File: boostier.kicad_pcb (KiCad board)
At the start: 2 copper layers, 7 parts, among them U1 TLV61070ADBV, U2 SN74LV1T126DBVR

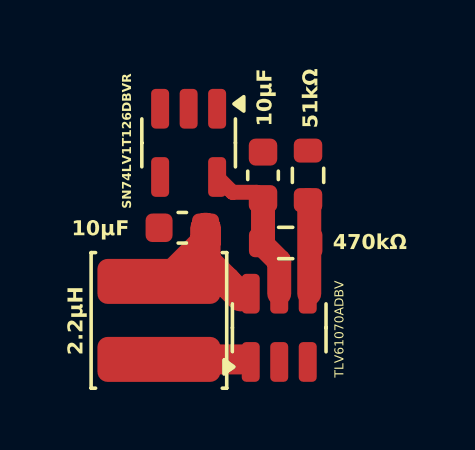
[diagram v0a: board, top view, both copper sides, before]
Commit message: Cleanup.
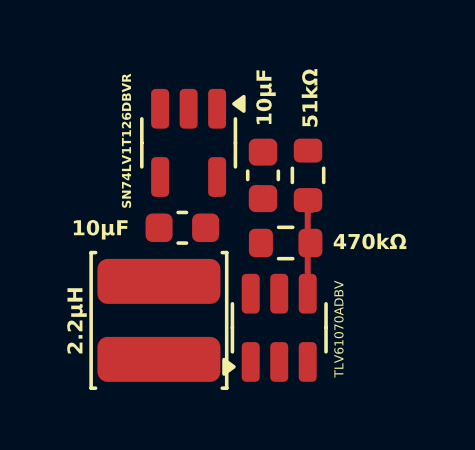
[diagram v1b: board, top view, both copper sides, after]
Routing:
- net RAW: track 7.58 -> 0.24 mm
- net 5V: track 5.28 -> 0.30 mm
- net BOOST_SW: track 2.75 -> 0.00 mm
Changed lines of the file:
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@@
-	)
-	(segment
-		(start 159.1025 98.97)
-		(end 160.415 97.6575)
-		(width 1)
-		(layer "F.Cu")
-		(net 1)
-	)
-	(segment
-		(start 158.86 98.97)
-		(end 161.09 98.97)
-		(width 1)
-		(layer "F.Cu")
-		(net 1)
-	)
-	(segment
-		(start 160.415 98.295)
-		(end 161.09 98.97)
-		(width 1)
-		(layer "F.Cu")
-		(net 1)
 	)
 	(segment
@@
 	)
 	(segment
-		(start 161.09 98.97)
-		(end 161.59 99.47)
-		(width 1)
-		(layer "F.Cu")
-		(net 1)
-	)
-	(segment
-		(start 160.415 97.6575)
-		(end 160.415 97.1825)
-		(width 1)
-		(layer "F.Cu")
-		(net 1)
-	)
-	(segment
-		(start 160.415 97.1825)
-		(end 160.415 98.295)
-		(width 1)
-		(layer "F.Cu")
-		(net 1)
-	)
-	(segment
-		(start 160.8 95.49)
-		(end 161.31 96)
-		(width 0.5)
-		(layer "F.Cu")
-		(net 3)
-	)
-	(segment
-		(start 162.33 97.62)
-		(end 162.26 97.69)
-		(width 0.8)
-		(layer "F.Cu")
-		(net 3)
-	)
-	(segment
-		(start 161.31 96)
-		(end 162.12 96)
-		(width 0.5)
-		(layer "F.Cu")
-		(net 3)
-	)
-	(segment
 		(start 162.12 96)
 		(end 162.33 96.21)
@@
 	)
 	(segment
-		(start 162.87 99.38)
-		(end 162.87 98.3)
-		(width 0.8)
+		(start 163.82 99.38)
+		(end 163.82 96.27)
+		(width 0.2)
 		(layer "F.Cu")
-		(net 3)
+		(net 7)
 	)
 	(segment
-		(start 162.33 96.21)
-		(end 162.33 97.62)
-		(width 0.8)
-		(layer "F.Cu")
-		(net 3)
-	)
-	(segment
-		(start 162.87 98.3)
-		(end 162.26 97.69)
-		(width 0.8)
-		(layer "F.Cu")
-		(net 3)
-	)
-	(segment
-		(start 163.871 96.301)
-		(end 163.871 99.38)
-		(width 0.8)
+		(start 163.82 96.27)
+		(end 163.83 96.26)
+		(width 0.2)
 		(layer "F.Cu")
 		(net 7)
@@
 		(net 7)
 	)
-	(segment
-		(start 158.86 101.57)
-		(end 161.61 101.57)
-		(width 1)
-		(layer "F.Cu")
-		(net 8)
-	)
 	(embedded_fonts no)
